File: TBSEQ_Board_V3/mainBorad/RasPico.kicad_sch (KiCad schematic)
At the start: 8 parts

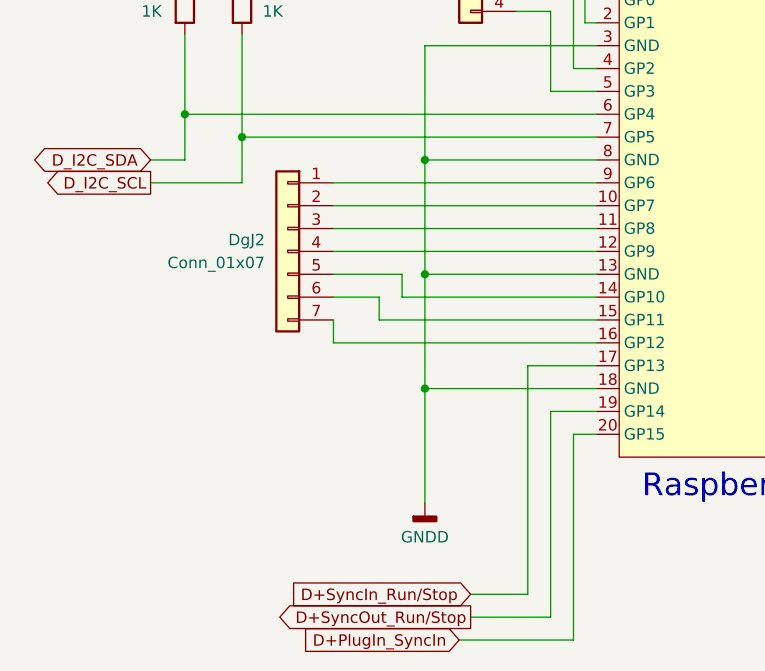
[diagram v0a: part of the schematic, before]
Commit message: BoardV3
ERCチェック済
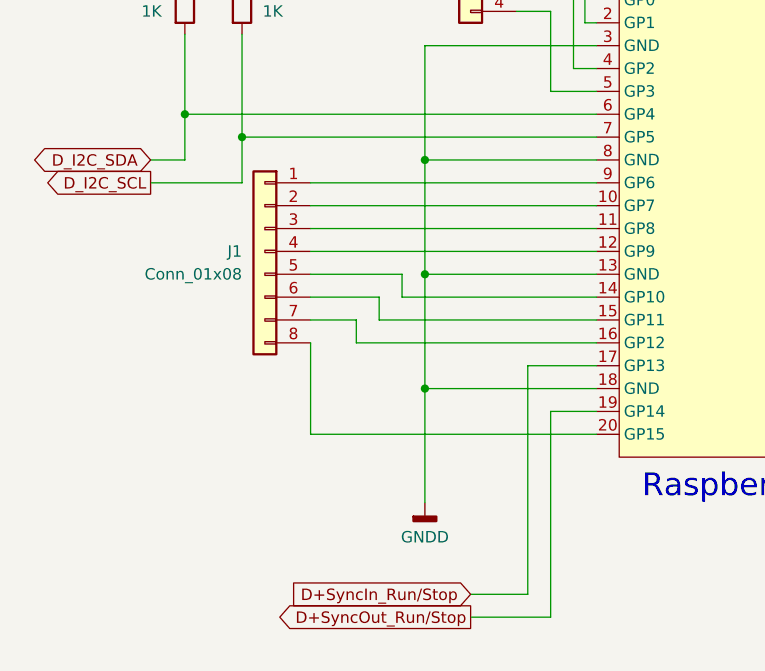
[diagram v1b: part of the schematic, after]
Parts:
- removed DgJ2: Conn_01x07, Connector_PinHeader_2.54mm:PinHeader_1x07_P2.54mm_Vertical, symbol Connector_Generic:Conn_01x07
- added J1: Conn_01x08, Connector_PinHeader_2.54mm:PinHeader_1x08_P2.54mm_Vertical, symbol Connector_Generic:Conn_01x08
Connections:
- net at DgU1.10 (GP7): now also J1.2 (Pin_2)
- net at DgU1.11 (GP8): now also J1.3 (Pin_3)
- net at DgU1.12 (GP9): now also J1.4 (Pin_4)
- net at DgU1.14 (GP10): now also J1.5 (Pin_5)
- net at DgU1.15 (GP11): now also J1.6 (Pin_6)
- net at DgU1.16 (GP12): now also J1.7 (Pin_7)
- net at DgU1.9 (GP6): now also J1.1 (Pin_1)
- net D+PlugIn_SyncIn: no longer names the net of DgU1.20 (GP15)
- net D+PlugIn_SyncIn: now also J1.8 (Pin_8)
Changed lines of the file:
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@@
+	(wire
+		(pts
+			(xy 62.23 121.92) (xy 62.23 124.46)
+		)
+		(stroke
+			(width 0)
+			(type default)
+		)
+	)
 	(wire
 		(pts
@@
 	(wire
 		(pts
-			(xy 59.69 124.46) (xy 59.69 121.92)
-		)
-		(stroke
-			(width 0)
-			(type default)
-		)
-	)
-	(wire
-		(pts
 			(xy 67.31 119.38) (xy 67.31 116.84)
 		)
@@
 	(wire
 		(pts
+			(xy 57.15 121.92) (xy 62.23 121.92)
+		)
+		(stroke
+			(width 0)
+			(type default)
+		)
+	)
+	(wire
+		(pts
 			(xy 80.01 80.01) (xy 88.9 80.01)
 		)
@@
 	(wire
 		(pts
-			(xy 59.69 106.68) (xy 88.9 106.68)
+			(xy 57.15 106.68) (xy 88.9 106.68)
 		)
 		(stroke
@@
 	(wire
 		(pts
-			(xy 59.69 109.22) (xy 88.9 109.22)
+			(xy 57.15 109.22) (xy 88.9 109.22)
 		)
 		(stroke
@@
 	(wire
 		(pts
-			(xy 86.36 157.48) (xy 86.36 134.62)
-		)
-		(stroke
-			(width 0)
-			(type default)
-		)
-	)
-	(wire
-		(pts
 			(xy 127 109.22) (xy 132.08 109.22)
 		)
@@
 	(wire
 		(pts
+			(xy 57.15 134.62) (xy 57.15 124.46)
+		)
+		(stroke
+			(width 0)
+			(type default)
+		)
+	)
+	(wire
+		(pts
 			(xy 186.69 72.39) (xy 186.69 76.2)
 		)
@@
 	(wire
 		(pts
-			(xy 86.36 134.62) (xy 88.9 134.62)
-		)
-		(stroke
-			(width 0)
-			(type default)
-		)
-	)
-	(wire
-		(pts
 			(xy 80.01 82.55) (xy 87.63 82.55)
 		)
@@
 	(wire
 		(pts
-			(xy 59.69 114.3) (xy 88.9 114.3)
+			(xy 57.15 114.3) (xy 88.9 114.3)
 		)
 		(stroke
@@
 	(wire
 		(pts
+			(xy 57.15 134.62) (xy 88.9 134.62)
+		)
+		(stroke
+			(width 0)
+			(type default)
+		)
+	)
+	(wire
+		(pts
 			(xy 43.18 90.17) (xy 43.18 99.06)
 		)
@@
 	(wire
 		(pts
-			(xy 73.66 157.48) (xy 86.36 157.48)
-		)
-		(stroke
-			(width 0)
-			(type default)
-		)
-	)
-	(wire
-		(pts
 			(xy 127 96.52) (xy 139.7 96.52)
 		)
@@
 	(wire
 		(pts
-			(xy 64.77 119.38) (xy 59.69 119.38)
+			(xy 64.77 119.38) (xy 57.15 119.38)
 		)
 		(stroke
@@
 	(wire
 		(pts
-			(xy 88.9 124.46) (xy 59.69 124.46)
+			(xy 88.9 124.46) (xy 62.23 124.46)
 		)
 		(stroke
@@
 	(wire
 		(pts
-			(xy 67.31 116.84) (xy 59.69 116.84)
+			(xy 67.31 116.84) (xy 57.15 116.84)
 		)
 		(stroke
@@
 	(wire
 		(pts
-			(xy 59.69 111.76) (xy 88.9 111.76)
+			(xy 57.15 111.76) (xy 88.9 111.76)
 		)
 		(stroke
@@
 		)
 	)
-	(global_label "D+PlugIn_SyncIn"
-		(shape input)
-		(at 73.66 157.48 180)
-		(fields_autoplaced yes)
-		(effects
-			(font
-				(size 1.27 1.27)
-			)
-			(justify right)
-		)
-		(property "Intersheetrefs" "${INTERSHEET_REFS}"
-			(at 54.7093 157.48 0)
-			(effects
-				(font
-					(size 1.27 1.27)
-				)
-				(justify right)
-				(hide yes)
-			)
-		)
-	)
 	(global_label "D+3.3V"
 		(shape output)
@@
 	)
 	(symbol
+		(lib_id "Connector_Generic:Conn_01x08")
+		(at 52.07 114.3 0)
+		(mirror y)
+		(unit 1)
+		(exclude_from_sim no)
+		(in_bom yes)
+		(on_board yes)
+		(dnp no)
+		(property "Reference" "J1"
+			(at 49.53 114.2999 0)
+			(effects
+				(font
+					(size 1.27 1.27)
+				)
+				(justify left)
+			)
+		)
+		(property "Value" "Conn_01x08"
+			(at 49.53 116.8399 0)
+			(effects
+				(font
+					(size 1.27 1.27)
+				)
+				(justify left)
+			)
+		)
+		(property "Footprint" "Connector_PinHeader_2.54mm:PinHeader_1x08_P2.54mm_Vertical"
+			(at 52.07 114.3 0)
+			(effects
+				(font
+					(size 1.27 1.27)
+				)
+				(hide yes)
+			)
+		)
+		(property "Datasheet" "~"
+			(at 52.07 114.3 0)
+			(effects
+				(font
+					(size 1.27 1.27)
+				)
+				(hide yes)
+			)
+		)
+		(property "Description" "Generic connector, single row, 01x08, script generated (kicad-library-utils/schlib/autogen/connector/)"
+			(at 52.07 114.3 0)
+			(effects
+				(font
+					(size 1.27 1.27)
+				)
+				(hide yes)
+			)
+		)
+		(pin "7"
+		)
+		(pin "1"
+		)
+		(pin "2"
+		)
+		(pin "6"
+		)
+		(pin "8"
+		)
+		(pin "3"
+		)
+		(pin "4"
+		)
+		(pin "5"
+		)
+		(instances
+			(project ""
+				(path "/83af791a-9776-40a7-82ad-9528ff7474b8/2a7aa622-1b89-4529-84ec-ef6853ee06a0"
+					(reference "J1")
+					(unit 1)
+				)
+			)
+		)
+	)
+	(symbol
 		(lib_id "Connector_Generic:Conn_01x06")
 		(at 172.72 95.25 0)
@@
 					(unit 1)
 				)
-			)
-		)
-	)
-	(symbol
-		(lib_id "Connector_Generic:Conn_01x07")
-		(at 54.61 114.3 0)
-		(mirror y)
-		(unit 1)
-		(exclude_from_sim no)
-		(in_bom yes)
-		(on_board yes)
-		(dnp no)
-		(property "Reference" "DgJ2"
-			(at 52.07 113.0299 0)
-			(effects
-				(font
-					(size 1.27 1.27)
-				)
-				(justify left)
-			)
-		)
-		(property "Value" "Conn_01x07"
-			(at 52.07 115.57 0)
-			(effects
-				(font
-					(size 1.27 1.27)
-				)
-				(justify left)
-			)
-		)
-		(property "Footprint" "Connector_PinHeader_2.54mm:PinHeader_1x07_P2.54mm_Vertical"
-			(at 54.61 114.3 0)
-			(effects
-				(font
-					(size 1.27 1.27)
-				)
-				(hide yes)
-			)
-		)
-		(property "Datasheet" "~"
-			(at 54.61 114.3 0)
-			(effects
-				(font
-					(size 1.27 1.27)
-				)
-				(hide yes)
-			)
-		)
-		(property "Description" "Generic connector, single row, 01x07, script generated (kicad-library-utils/schlib/autogen/connector/)"
-			(at 54.61 114.3 0)
-			(effects
-				(font
-					(size 1.27 1.27)
-				)
-				(hide yes)
-			)
-		)
-		(pin "3"
-		)
-		(pin "6"
-		)
-		(pin "1"
-		)
-		(pin "4"
-		)
-		(pin "7"
-		)
-		(pin "5"
-		)
-		(pin "2"
-		)
-		(instances
-			(project "mainBorad"
-				(path "/83af791a-9776-40a7-82ad-9528ff7474b8/2a7aa622-1b89-4529-84ec-ef6853ee06a0"
-					(reference "DgJ2")
-					(unit 1)
-				)

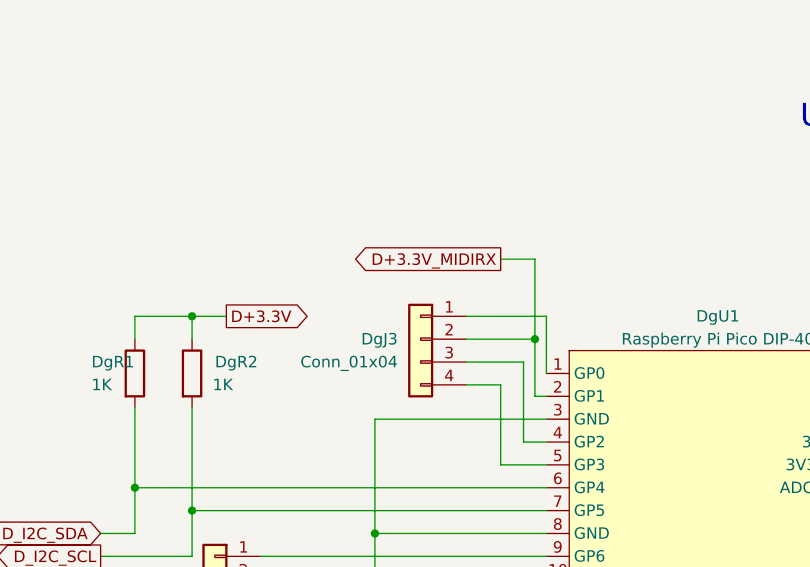
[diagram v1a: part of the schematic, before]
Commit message: V3Board
アートワーク中
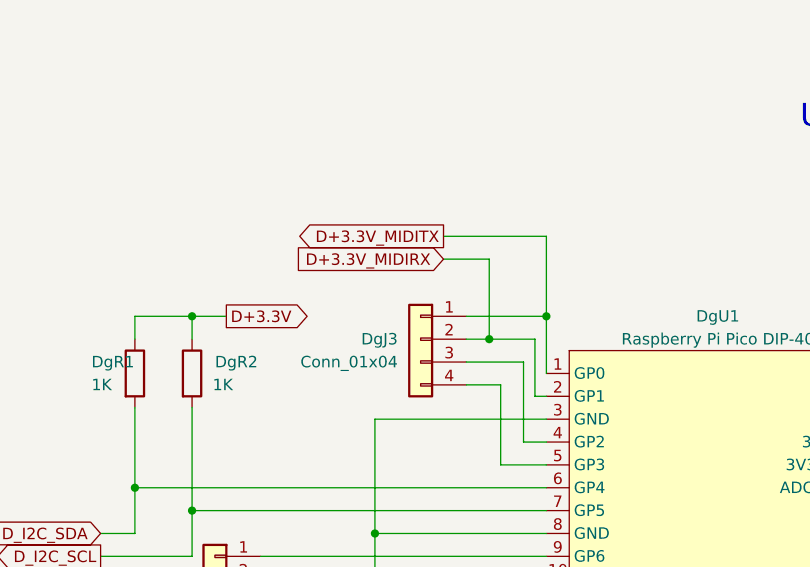
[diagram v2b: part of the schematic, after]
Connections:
- net D+3.3V_MIDITX: now reaches DgJ3.1 (Pin_1), DgU1.1 (GP0)
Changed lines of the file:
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@@
+	)
+	(junction
+		(at 88.9 80.01)
+		(diameter 0)
+		(color 0 0 0 0)
 	)
 	(junction
@@
 	)
 	(junction
+		(at 82.55 82.55)
+		(diameter 0)
+		(color 0 0 0 0)
+	)
+	(junction
 		(at 49.53 80.01)
 		(diameter 0)
@@
 	)
 	(junction
-		(at 87.63 82.55)
-		(diameter 0)
-		(color 0 0 0 0)
-	)
-	(junction
 		(at 156.21 74.93)
 		(diameter 0)
@@
 	(wire
 		(pts
-			(xy 87.63 73.66) (xy 83.82 73.66)
+			(xy 82.55 73.66) (xy 77.47 73.66)
 		)
 		(stroke
@@
 	(wire
 		(pts
+			(xy 77.47 71.12) (xy 88.9 71.12)
+		)
+		(stroke
+			(width 0)
+			(type default)
+		)
+	)
+	(wire
+		(pts
 			(xy 49.53 90.17) (xy 49.53 101.6)
 		)
@@
 	(wire
 		(pts
-			(xy 80.01 82.55) (xy 87.63 82.55)
+			(xy 80.01 82.55) (xy 82.55 82.55)
 		)
 		(stroke
@@
 	(wire
 		(pts
+			(xy 82.55 82.55) (xy 87.63 82.55)
+		)
+		(stroke
+			(width 0)
+			(type default)
+		)
+	)
+	(wire
+		(pts
 			(xy 43.18 90.17) (xy 43.18 99.06)
 		)
@@
 	(wire
 		(pts
-			(xy 87.63 82.55) (xy 87.63 73.66)
+			(xy 82.55 82.55) (xy 82.55 73.66)
+		)
+		(stroke
+			(width 0)
+			(type default)
+		)
+	)
+	(wire
+		(pts
+			(xy 88.9 71.12) (xy 88.9 80.01)
 		)
 		(stroke
@@
 	)
 	(global_label "D+3.3V_MIDIRX"
-		(shape output)
-		(at 83.82 73.66 180)
+		(shape input)
+		(at 77.47 73.66 180)
 		(fields_autoplaced yes)
 		(effects
@@
 		)
 		(property "Intersheetrefs" "${INTERSHEET_REFS}"
-			(at 72.0053 73.66 0)
+			(at 65.6553 73.66 0)
 			(effects
 				(font
@@
 		(property "Intersheetrefs" "${INTERSHEET_REFS}"
 			(at 52.8346 152.4 0)
+			(effects
+				(font
+					(size 1.27 1.27)
+				)
+				(justify right)
+				(hide yes)
+			)
+		)
+	)
+	(global_label "D+3.3V_MIDITX"
+		(shape output)
+		(at 77.47 71.12 180)
+		(fields_autoplaced yes)
+		(effects
+			(font
+				(size 1.27 1.27)
+			)
+			(justify right)
+		)
+		(property "Intersheetrefs" "${INTERSHEET_REFS}"
+			(at 65.6553 71.12 0)
 			(effects
 				(font
@@
 			)
 		)
+		(property "Sim.Library" ""
+			(at 107.95 109.22 0)
+			(effects
+				(font
+					(size 1.27 1.27)
+				)
+				(hide yes)
+			)
+		)
+		(property "Sim.Name" ""
+			(at 107.95 109.22 0)
+			(effects
+				(font
+					(size 1.27 1.27)
+				)
+				(hide yes)
+			)
+		)
 		(pin "32"
 		)
@@
 			)
 		)
+		(property "Sim.Library" ""
+			(at 180.34 111.76 0)
+			(effects
+				(font
+					(size 1.27 1.27)
+				)
+				(hide yes)
+			)
+		)
+		(property "Sim.Name" ""
+			(at 180.34 111.76 0)
+			(effects
+				(font
+					(size 1.27 1.27)
+				)
+				(hide yes)
+			)
+		)
 		(pin "3"
 		)
@@
 		)
 		(property "Description" "-3.7A Id, -20V Vds, 65mOhm Rds, P-Channel HEXFET Power MOSFET, SOT-23"
+			(at 135.89 77.47 0)
+			(effects
+				(font
+					(size 1.27 1.27)
+				)
+				(hide yes)
+			)
+		)
+		(property "Sim.Library" ""
+			(at 135.89 77.47 0)
+			(effects
+				(font
+					(size 1.27 1.27)
+				)
+				(hide yes)
+			)
+		)
+		(property "Sim.Name" ""
 			(at 135.89 77.47 0)
 			(effects
@@
 			)
 		)
+		(property "Sim.Library" ""
+			(at 74.93 82.55 0)
+			(effects
+				(font
+					(size 1.27 1.27)
+				)
+				(hide yes)
+			)
+		)
+		(property "Sim.Name" ""
+			(at 74.93 82.55 0)
+			(effects
+				(font
+					(size 1.27 1.27)
+				)
+				(hide yes)
+			)
+		)
 		(pin "4"
 		)
@@
 		)
 		(property "Description" "Resistor"
+			(at 49.53 86.36 0)
+			(effects
+				(font
+					(size 1.27 1.27)
+				)
+				(hide yes)
+			)
+		)
+		(property "Sim.Library" ""
+			(at 49.53 86.36 0)
+			(effects
+				(font
+					(size 1.27 1.27)
+				)
+				(hide yes)
+			)
+		)
+		(property "Sim.Name" ""
 			(at 49.53 86.36 0)
 			(effects
@@
 			)
 		)
+		(property "Sim.Library" ""
+			(at 52.07 114.3 0)
+			(effects
+				(font
+					(size 1.27 1.27)
+				)
+				(hide yes)
+			)
+		)
+		(property "Sim.Name" ""
+			(at 52.07 114.3 0)
+			(effects
+				(font
+					(size 1.27 1.27)
+				)
+				(hide yes)
+			)
+		)
 		(pin "7"
 		)
@@
 			)
 		)
+		(property "Sim.Library" ""
+			(at 172.72 95.25 0)
+			(effects
+				(font
+					(size 1.27 1.27)
+				)
+				(hide yes)
+			)
+		)
+		(property "Sim.Name" ""
+			(at 172.72 95.25 0)
+			(effects
+				(font
+					(size 1.27 1.27)
+				)
+				(hide yes)
+			)
+		)
 		(pin "2"
 		)
@@
 			(at 43.18 86.36 0)
 			(effects
+				(font
+					(size 1.27 1.27)
+				)
+				(hide yes)
+			)
+		)
+		(property "Sim.Library" ""
+			(at 43.18 86.36 0)
+			(effects
+				(font
+					(size 1.27 1.27)
+				)
+				(hide yes)
+			)
+		)
+		(property "Sim.Name" ""
+			(at 43.18 86.36 0)
+			(effects
